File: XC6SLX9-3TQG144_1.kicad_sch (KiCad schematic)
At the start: 11 parts, among them U1 XC6SLX9-3TQG144, U2 SST25VF040B-50-4C-SAF-T

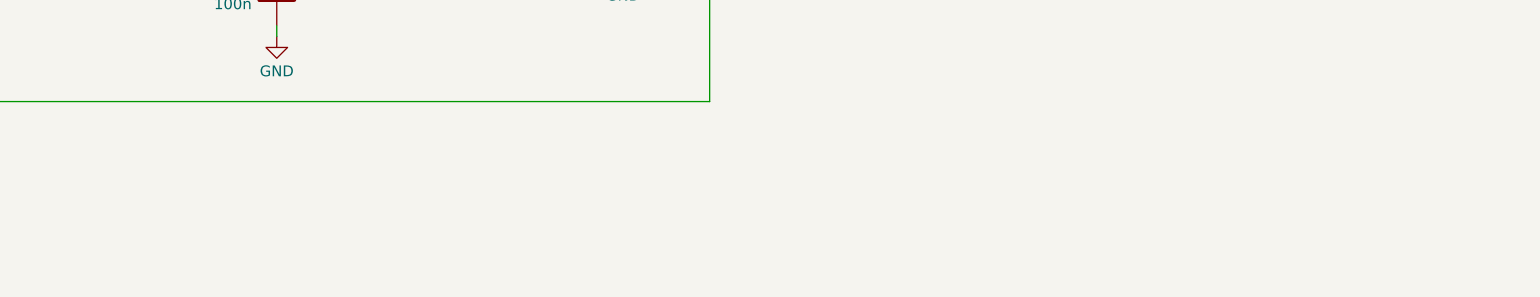
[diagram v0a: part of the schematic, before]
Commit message: first draft - ready for review
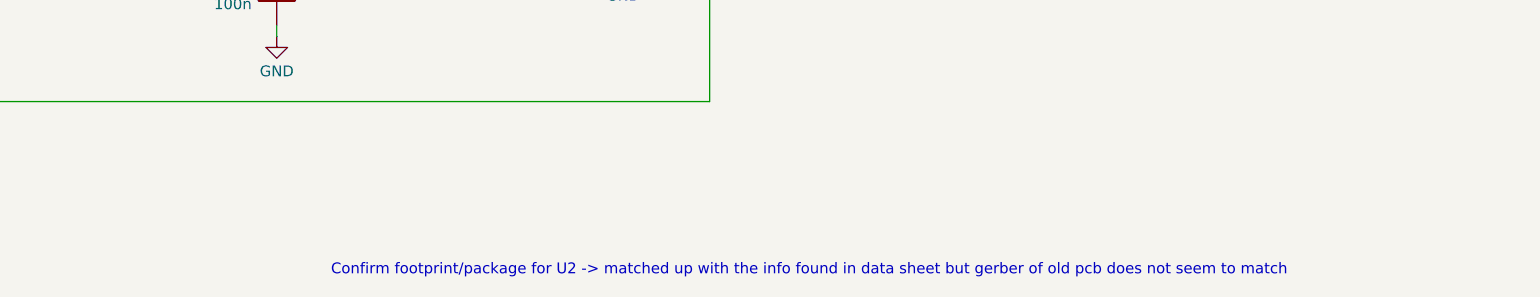
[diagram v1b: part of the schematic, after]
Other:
- note added: "Confirm footprint/package for U2 -> matched up with the info found in data sheet but gerber of old pcb does not seem to match"
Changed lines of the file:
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@@
+		)
+	)
+	(text "Confirm footprint/package for U2 -> matched up with the info found in data sheet but gerber of old pcb does not seem to match"
+		(exclude_from_sim no)
+		(at 174.244 215.392 0)
+		(effects
+			(font
+				(size 1.27 1.27)
+			)
 		)
 	)
